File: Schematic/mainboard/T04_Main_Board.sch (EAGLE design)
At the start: 14 parts, among them IC1 7805DT, J1 AVR_SPI_PRG_6PTH, U1 ATMEGA328P_PDIP

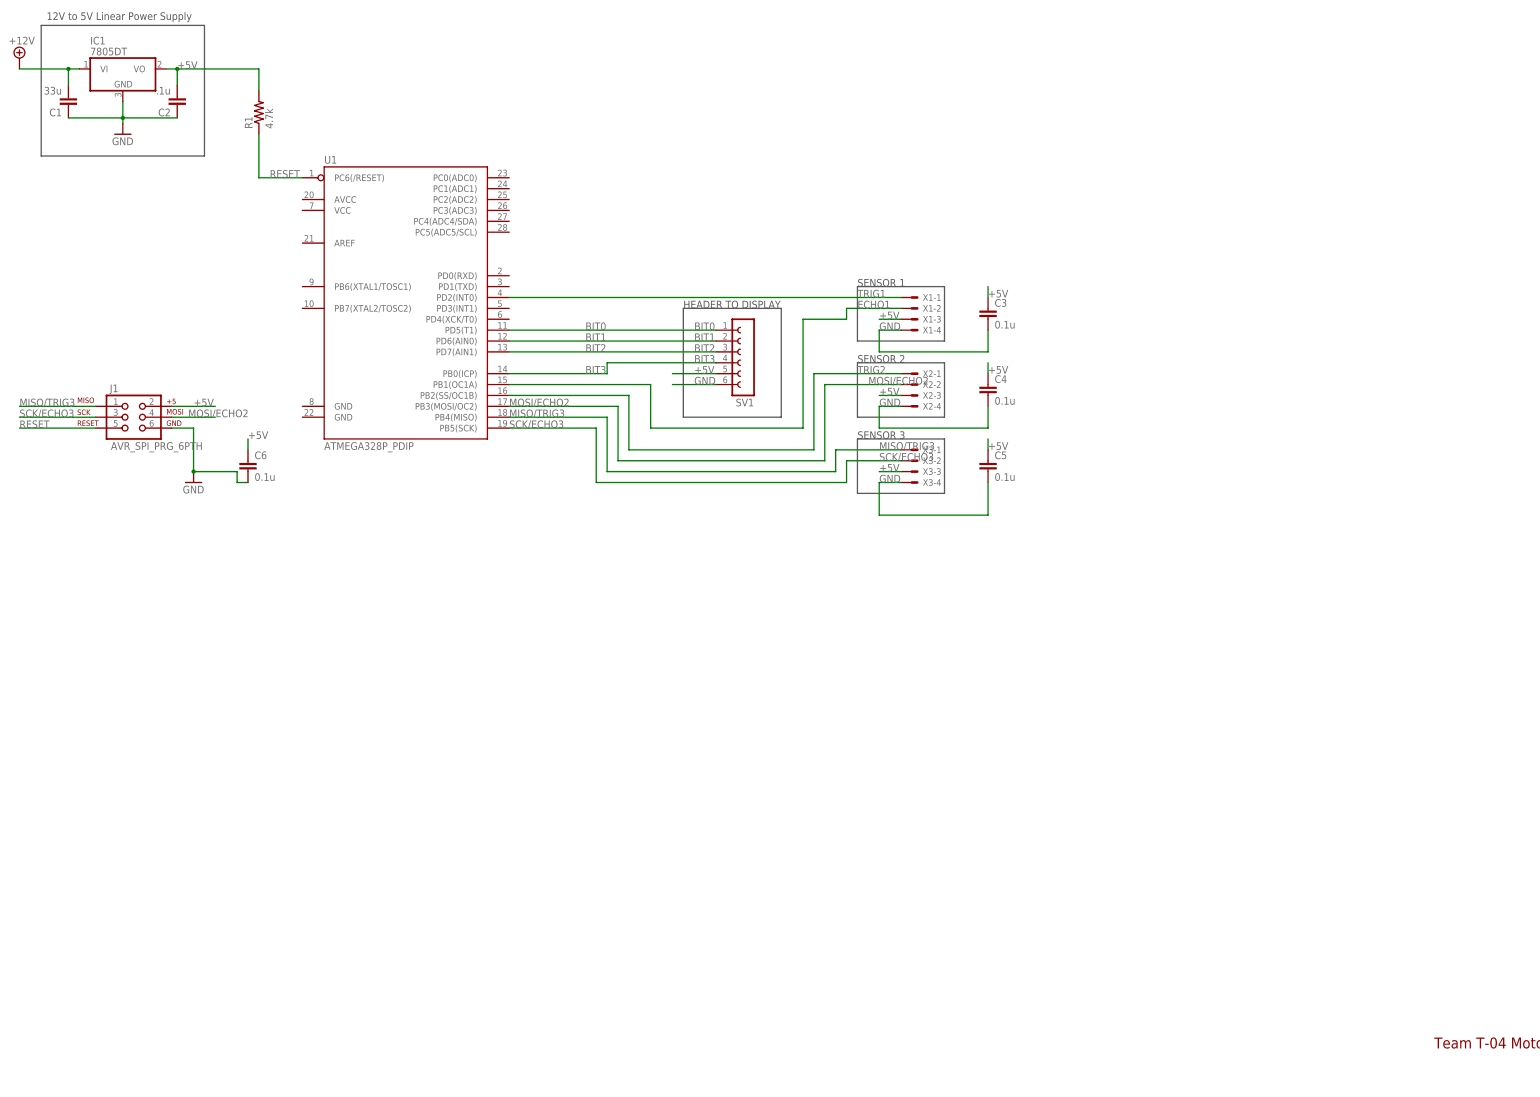
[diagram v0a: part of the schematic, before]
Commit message: Mainboard Update and Prototype_rev4 update
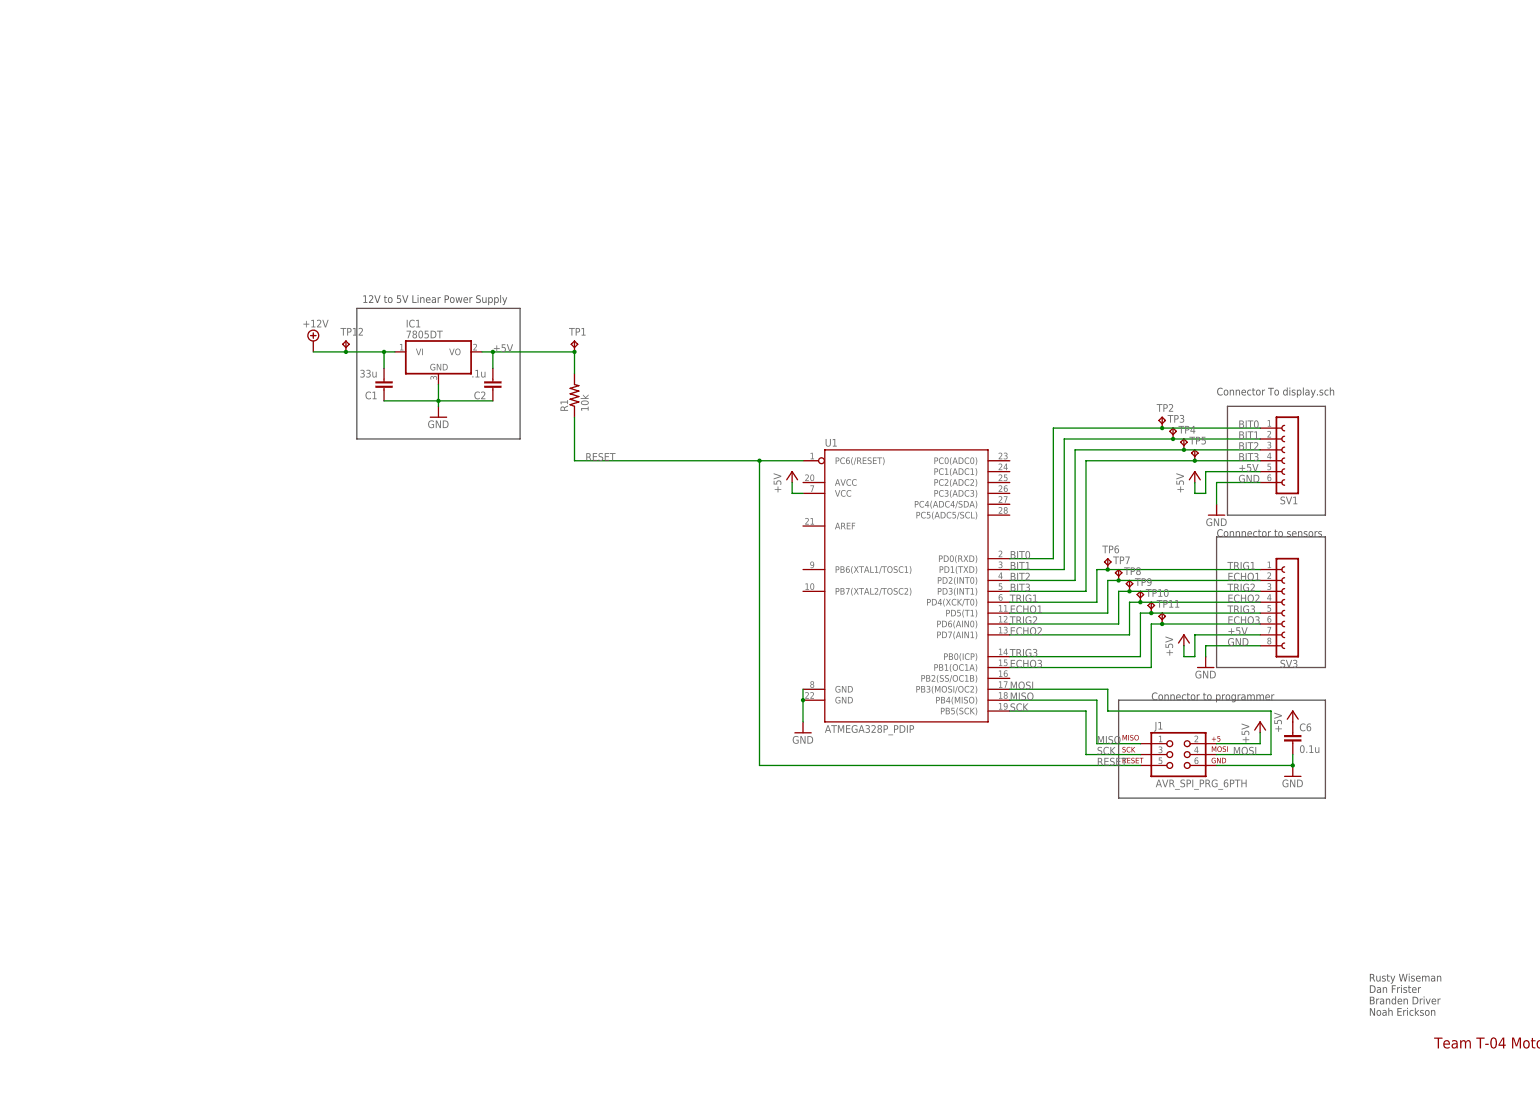
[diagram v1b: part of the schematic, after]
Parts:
- removed C3, C4, C5: 0.1u, rcl:C-EUC3225
- removed X1, X2, X3: (no value), con-molex:KK-156-4
- added SV3: (no value), con-lsta:FE08-1
- added TP1, TP10, TP11, TP12, TP2, TP3, TP4, TP5, TP6, TP7, TP8, TP9: TPB1,27, testpad:TPB1,27
- C6: device rcl:C-EUC3225 -> rcl:C-EU025-024X044
- R1: value 4.7k -> 10k; device rcl:R-US_0414/5V -> rcl:R-US_M2309
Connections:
- removed net MISO/TRIG3: J1.1, U1.PB4(MISO), X3-1.S
- removed net MOSI/ECHO2: J1.4, U1.PB3(MOSI/OC2), X2-2.S
- removed net SCK/ECHO3: J1.3, U1.PB5(SCK), X3-2.S
- new net ECHO2: SV3.4, TP9.TP, U1.PD7(AIN1)
- new net ECHO3: SV3.6, TP11.TP, U1.PB1(OC1A)
- new net MISO: J1.1, U1.PB4(MISO)
- new net MOSI: J1.4, U1.PB3(MOSI/OC2)
- new net SCK: J1.3, U1.PB5(SCK)
- new net TRIG3: SV3.5, TP10.TP, U1.PB0(ICP)
- net +12V: now also TP12.TP
- net +5V: now also SV3.7, TP1.TP, U1.VCC; no longer C3.1, C4.1, C5.1, X1-3.S, X2-3.S, X3-3.S
- net BIT0: now also TP2.TP, U1.PD0(RXD); no longer U1.PD5(T1)
- net BIT1: now also TP3.TP, U1.PD1(TXD); no longer U1.PD6(AIN0)
- net BIT2: now also TP4.TP, U1.PD2(INT0); no longer U1.PD7(AIN1)
- net BIT3: now also TP5.TP, U1.PD3(INT1); no longer U1.PB0(ICP)
- net ECHO1: now also SV3.2, TP7.TP, U1.PD5(T1); no longer U1.PB1(OC1A), X1-2.S
- net GND: now also SV3.8, U1.GND@1, U1.GND@2; no longer C3.2, C4.2, C5.2, X1-4.S, X2-4.S, X3-4.S
- net TRIG1: now also SV3.1, TP6.TP, U1.PD4(XCK/T0); no longer U1.PD2(INT0), X1-1.S
- net TRIG2: now also SV3.3, TP8.TP, U1.PD6(AIN0); no longer U1.PB2(SS/OC1B), X2-1.S
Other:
- note added: "Connector To display.sch"
- note added: "Connector to programmer"
- note added: "Connnector to sensors"
- note added: "Rusty Wiseman Dan Frister Branden Driver Noah Erickson"
- note removed: "HEADER TO DISPLAY"
- note removed: "SENSOR 1"
- note removed: "SENSOR 2"
- note removed: "SENSOR 3"
- moved on the sheet: C1, C2, C6, IC1, J1, R1, SV1, U1
